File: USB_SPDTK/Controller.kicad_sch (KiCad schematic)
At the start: 40 parts, among them J1 USB_B_Micro, J2 TagConnectTC2050, J3 Conn_02x08_Odd_Even, SW1 SW_Push, SW2 SW_Push, U3 STM32F411RETx, U3 ULN2003ADR, U4 93LC66AT-IOT, Y1 16M 20pF 3225

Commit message: Update LCSC for pushbuttons
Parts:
- SW1, SW2: LCSC C2800965 -> C118141

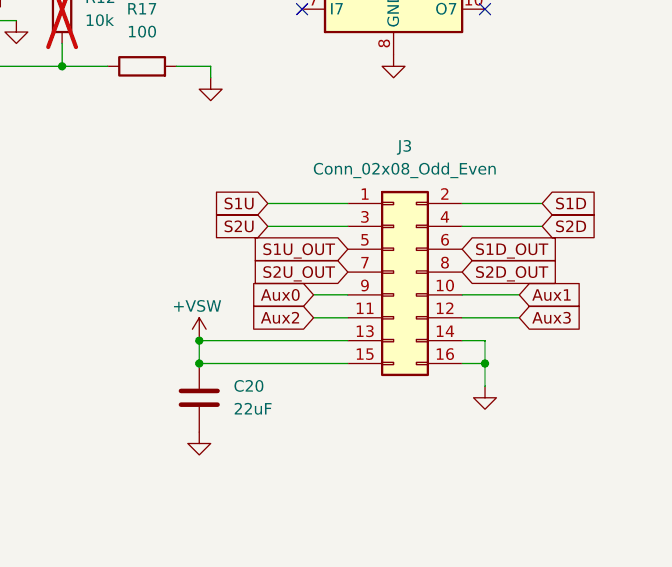
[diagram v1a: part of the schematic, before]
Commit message: Final submission to JLCPCB
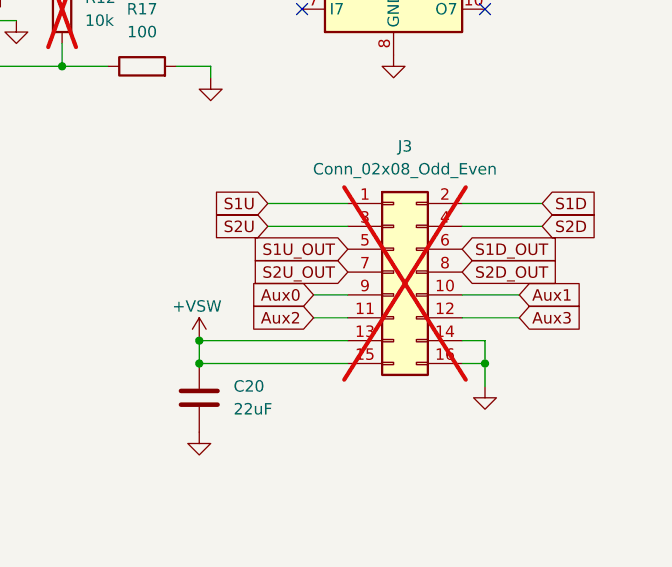
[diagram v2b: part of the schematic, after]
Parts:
- J3: now not fitted
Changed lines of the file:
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@@
 		(in_bom yes)
 		(on_board yes)
-		(dnp no)
+		(dnp yes)
 		(fields_autoplaced yes)
 		(property "Reference" "J3"

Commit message: .
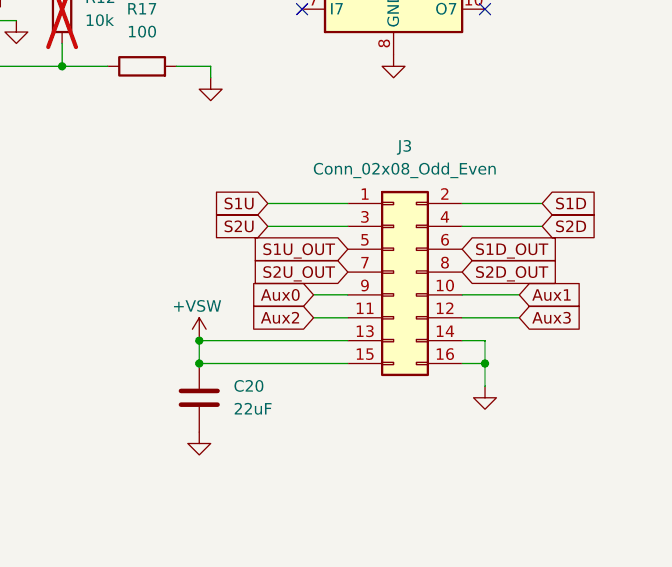
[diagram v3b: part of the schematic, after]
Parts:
- J3: now fitted
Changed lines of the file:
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@@
 		(in_bom yes)
 		(on_board yes)
-		(dnp yes)
+		(dnp no)
 		(fields_autoplaced yes)
 		(property "Reference" "J3"
